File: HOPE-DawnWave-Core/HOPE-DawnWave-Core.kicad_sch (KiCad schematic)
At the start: 37 parts, among them J1 USB_C_Receptacle_USB2.0_16P, SW1 RST, SW2 BOOT, U1 TLV62569DRL, U2 USBLC6-2P6, U3 ESP32-C6-WROOM-1

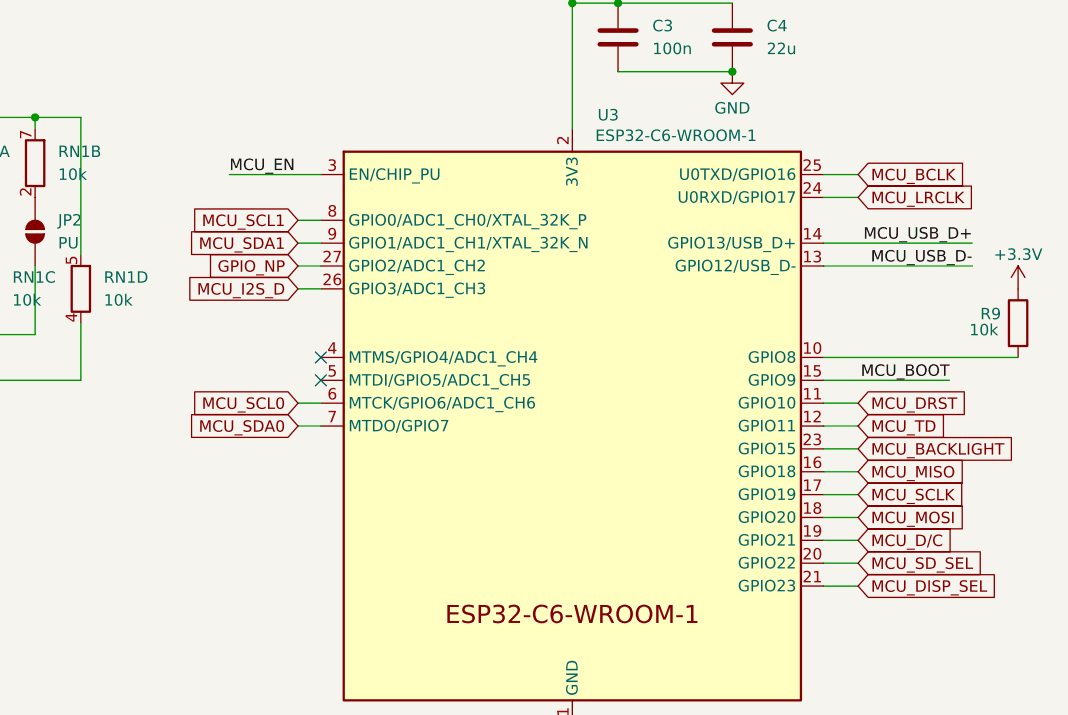
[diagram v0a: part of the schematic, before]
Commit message: big progress oops
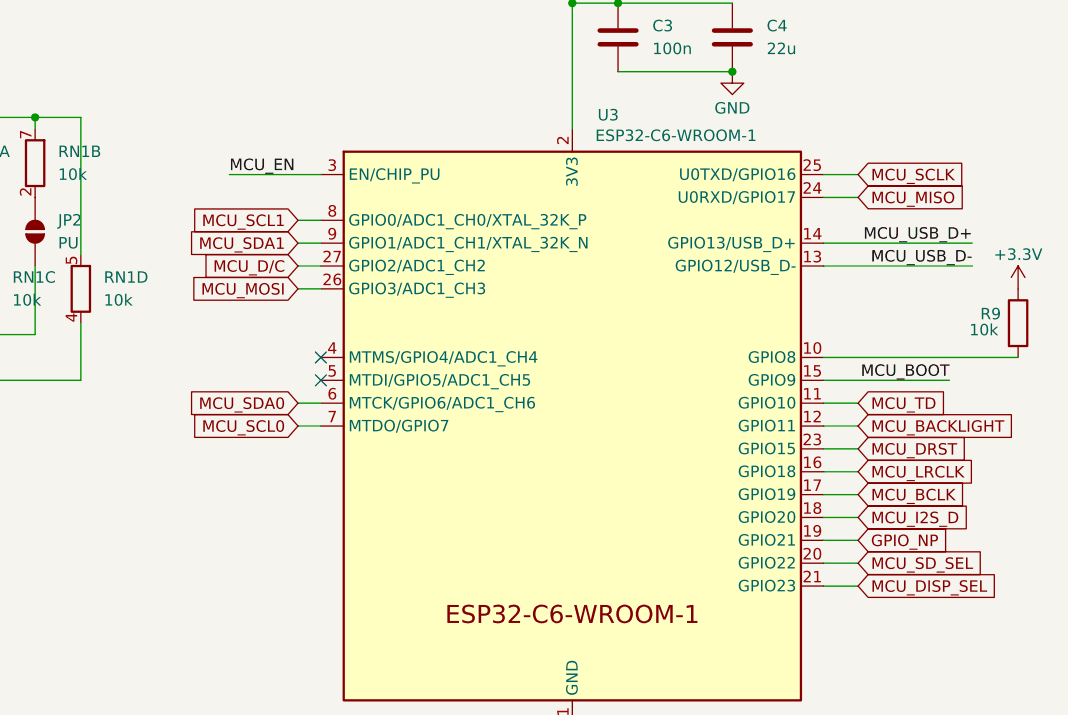
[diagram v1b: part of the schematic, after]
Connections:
- net GPIO_NP: now also U3.19 (GPIO21); no longer U3.27 (GPIO2/ADC1_CH2)
- net MCU_BACKLIGHT: now also U3.12 (GPIO11); no longer U3.23 (GPIO15)
- net MCU_BCLK: now also U3.17 (GPIO19); no longer U3.25 (U0TXD/GPIO16)
- net MCU_DRST: now also U3.23 (GPIO15); no longer U3.11 (GPIO10)
- net MCU_D/C: now also U3.27 (GPIO2/ADC1_CH2); no longer U3.19 (GPIO21)
- net MCU_I2S_D: now also U3.18 (GPIO20); no longer U3.26 (GPIO3/ADC1_CH3)
- net MCU_LRCLK: now also U3.16 (GPIO18); no longer U3.24 (U0RXD/GPIO17)
- net MCU_MISO: now also U3.24 (U0RXD/GPIO17); no longer U3.16 (GPIO18)
- net MCU_MOSI: now also U3.26 (GPIO3/ADC1_CH3); no longer U3.18 (GPIO20)
- net MCU_SCL0: now also U3.7 (MTDO/GPIO7); no longer U3.6 (MTCK/GPIO6/ADC1_CH6)
- net MCU_SCLK: now also U3.25 (U0TXD/GPIO16); no longer U3.17 (GPIO19)
- net MCU_SDA0: now also U3.6 (MTCK/GPIO6/ADC1_CH6); no longer U3.7 (MTDO/GPIO7)
- net MCU_TD: now also U3.11 (GPIO10); no longer U3.12 (GPIO11)
